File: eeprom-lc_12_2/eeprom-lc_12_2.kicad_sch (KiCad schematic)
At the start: 9 parts, among them J1 Conn_02x05_Pin

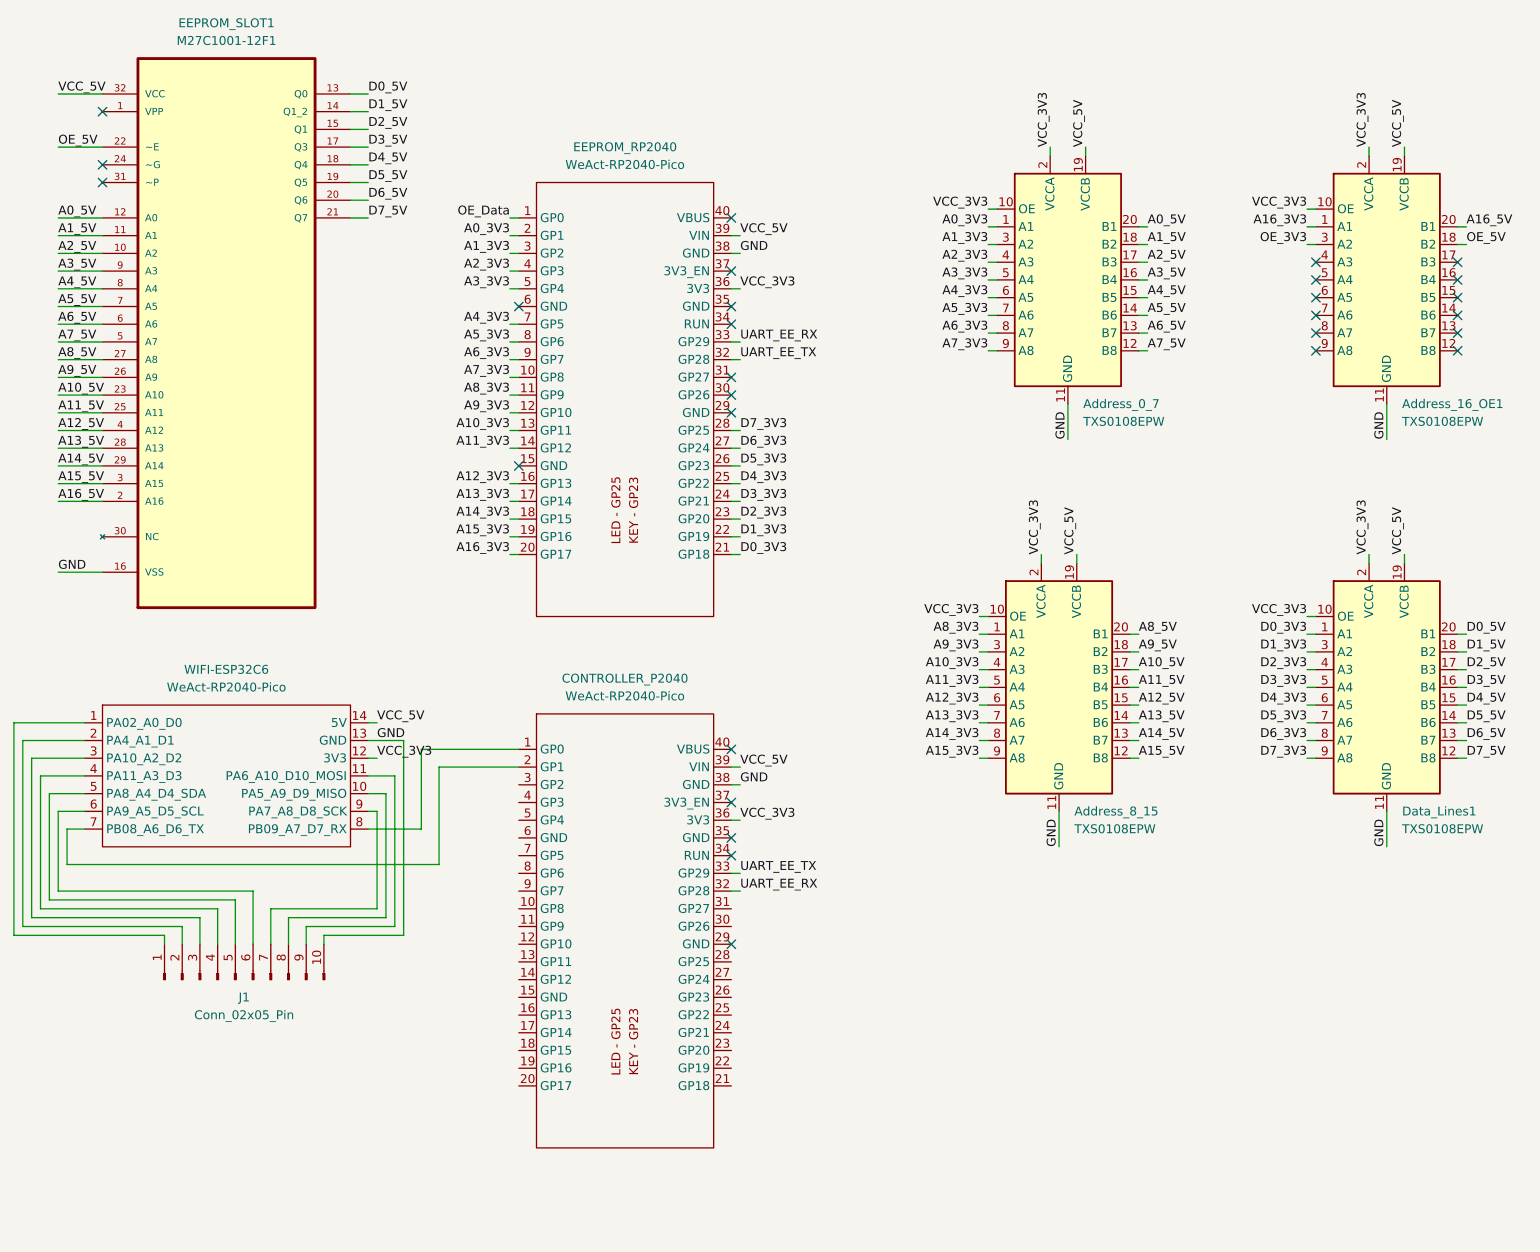
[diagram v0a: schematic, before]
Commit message: More work on pcb
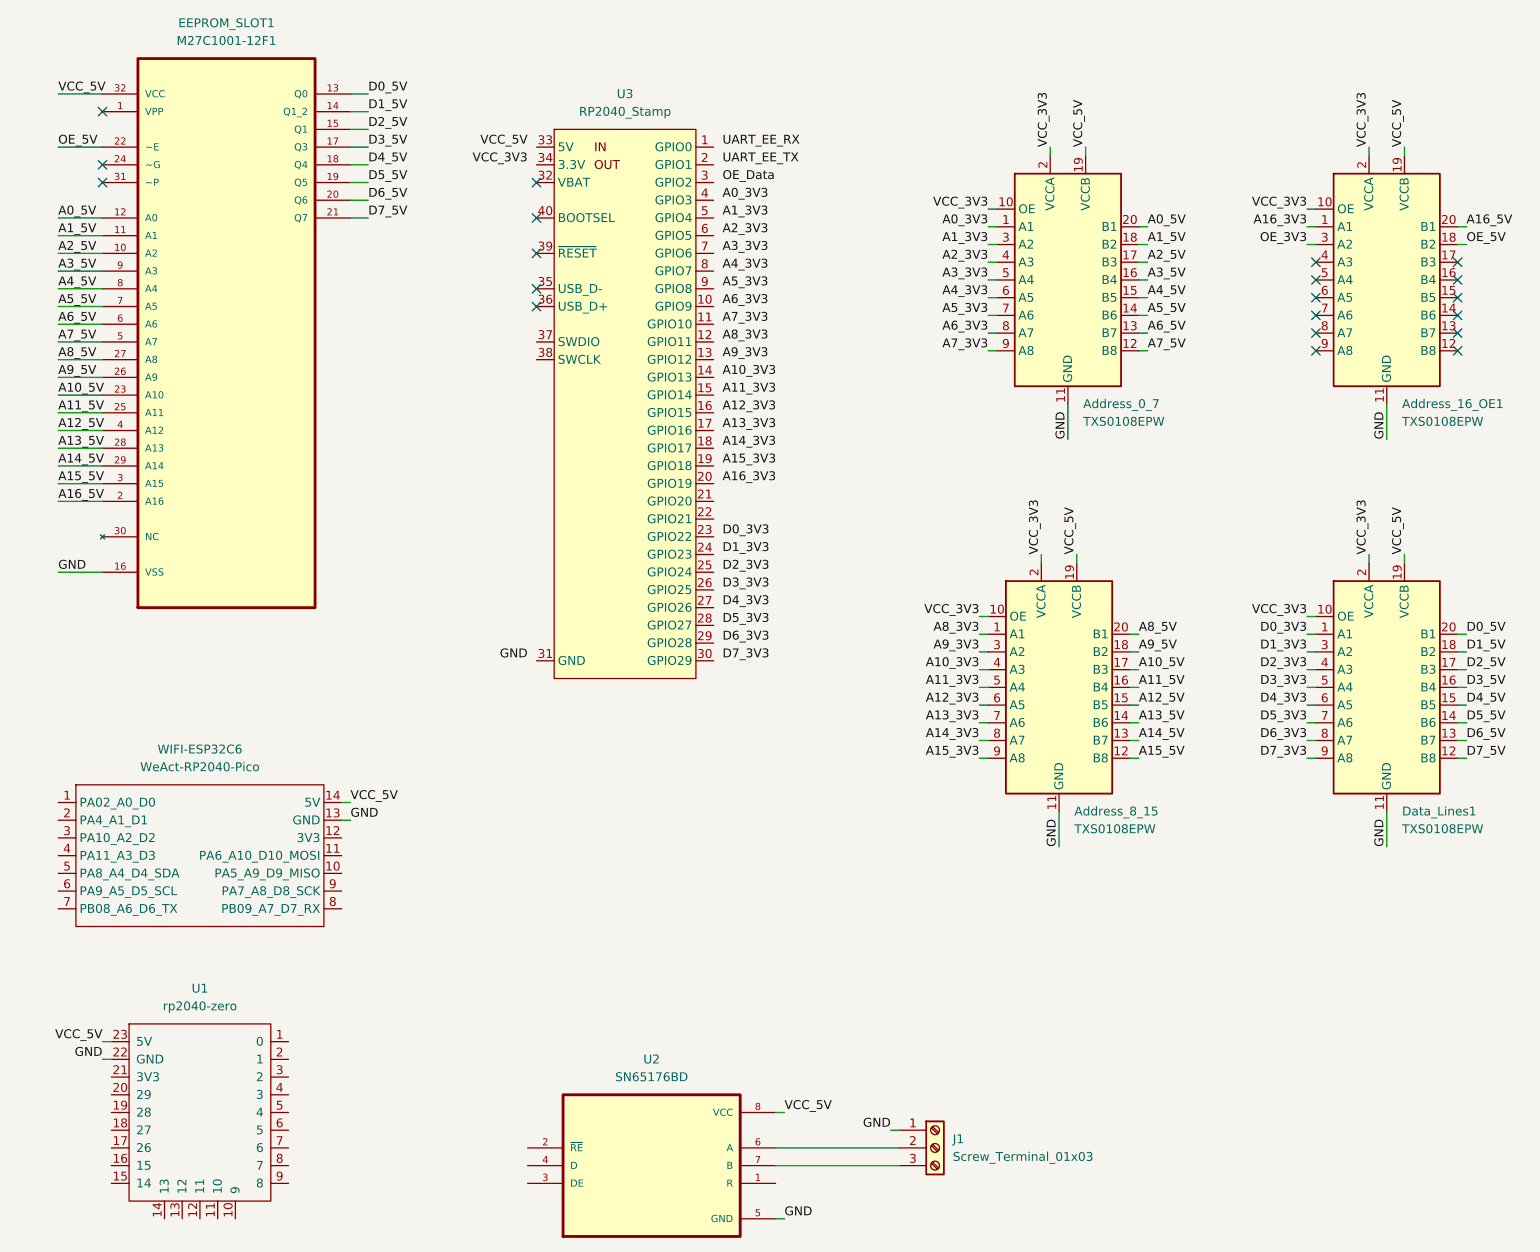
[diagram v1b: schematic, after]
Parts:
- removed CONTROLLER_P2040, EEPROM_RP2040: WeAct-RP2040-Pico, WeAct-RP2040-Pico:WeAct-RP2040-Pico, symbol WeAct-RP2040-Pico:WeAct-RP2040-Pico
- removed J1: Conn_02x05_Pin, Connector_PinHeader_2.00mm:PinHeader_2x05_P2.00mm_Vertical, symbol Connector:Conn_01x10_Pin
- added J1: Screw_Terminal_01x03, TerminalBlock:TerminalBlock_Xinya_XY308-2.54-3P_1x03_P2.54mm_Horizontal, symbol Connector:Screw_Terminal_01x03
- added U1: rp2040-zero, kleeb-mcu:rp2040-zero-smd, symbol kleeb-mcu:rp2040-zero
- added U2: SN65176BD, SN65176BD:SOIC127P599X175-8N, symbol SN65176BD:SN65176BD
- added U3: RP2040_Stamp, RP2040_Stamp:RP2040_Stamp_SMD, symbol RP2040_Stamp:RP2040_Stamp
- WIFI-ESP32C6: footprint XIAO_PCB:MOUDLE14P-2.54-21X17.8MM -> XIAO_PCB:MOUDLE14P-SMD-2.54-21X17.8MM
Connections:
- net GND: now also J1.1 (Pin_1), U1.22 (GND), U2.5 (GND)
- net VCC_3V3: no longer WIFI-ESP32C6.12 (3V3)
- net VCC_5V: now also U1.23 (5V), U2.8 (VCC)
- new net: J1.2 (Pin_2), U2.6 (A)
- new net: J1.3 (Pin_3), U2.7 (B)
- no-connect marks 29 -> 20
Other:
- moved on the sheet: WIFI-ESP32C6
